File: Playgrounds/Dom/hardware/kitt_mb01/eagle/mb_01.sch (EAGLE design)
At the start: 50 parts, among them CON1 ARDUINO_UNO, CON2 KITT.DB01, IC1 LA5744TP, IC2.00 BQ24266RGET

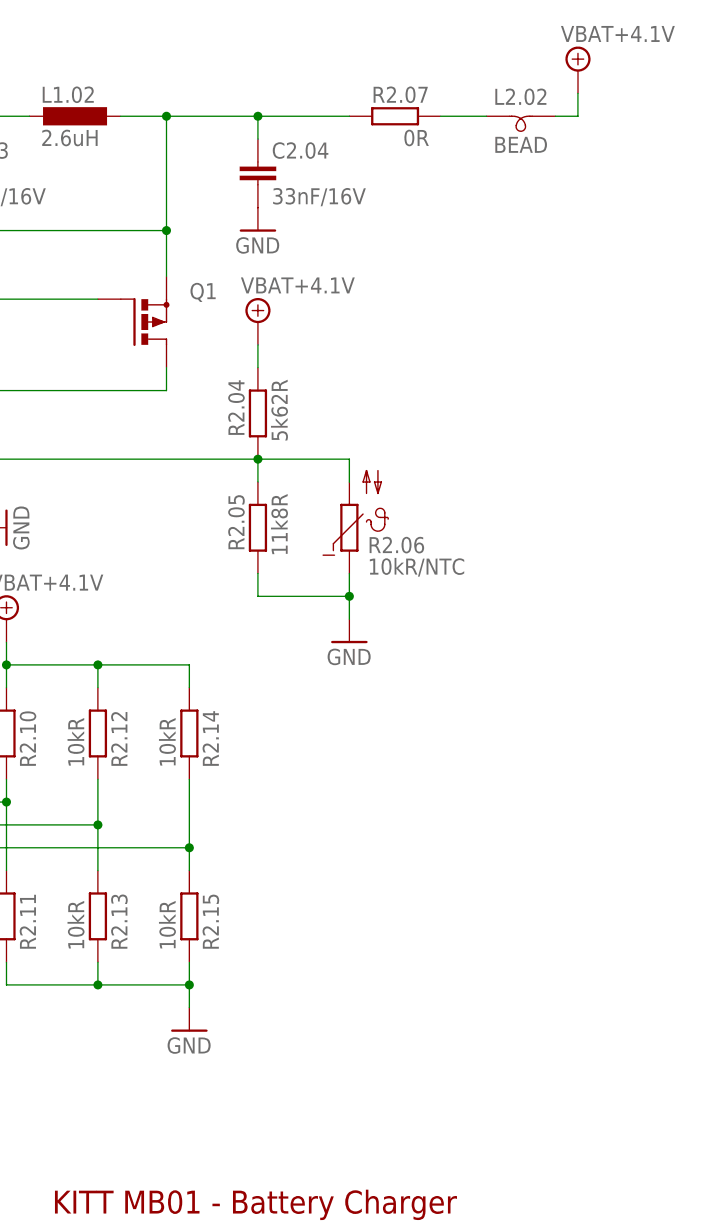
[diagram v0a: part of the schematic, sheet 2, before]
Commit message: did some more work on copying the charger layout
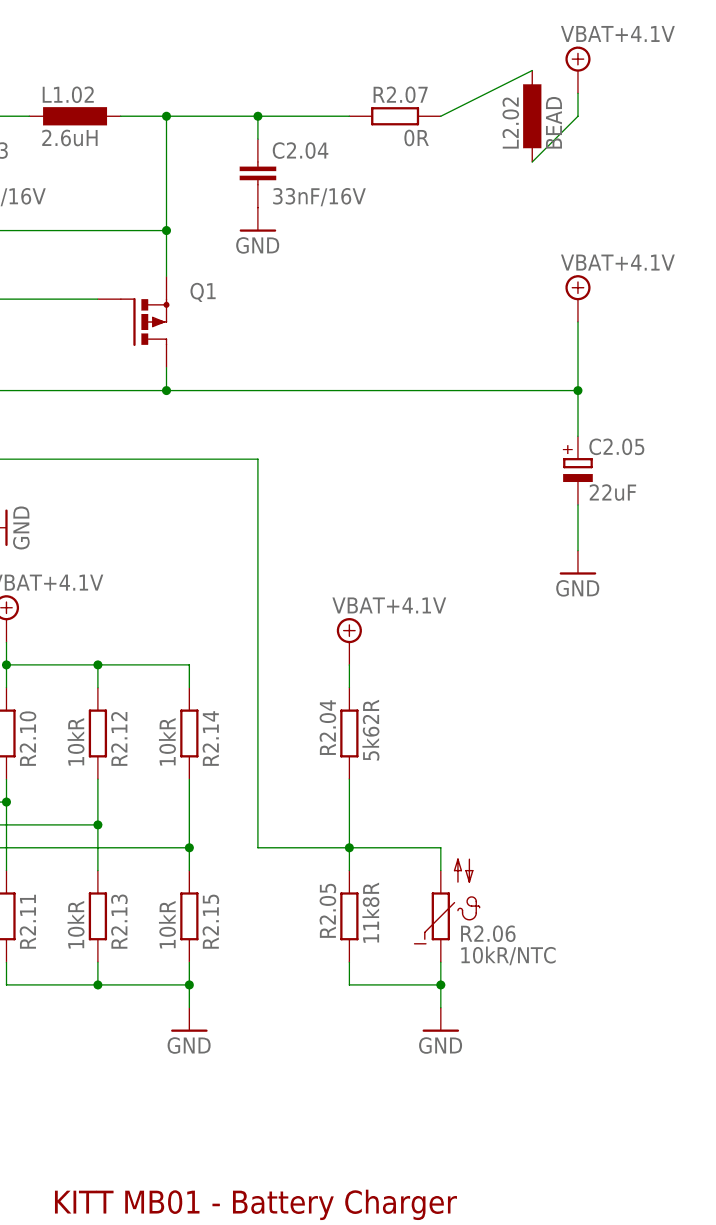
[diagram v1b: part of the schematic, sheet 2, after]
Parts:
- added C2.05: 22uF, rcl:CPOL-EUA/3216-18R
- C2.03: device rcl:C-EUC0805 -> rcl:C-EUC0603
- L2.02: device inductor-neosid:SM-B5 -> rcl:L-EUL2012C
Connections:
- removed net N$17: IC2.00PINS.BAT@1, IC2.00PINS.BAT@2, Q1.D
- net +4.1V: now also C2.05.+, IC2.00PINS.BAT@1, IC2.00PINS.BAT@2, Q1.D
- net GND: now also C2.05.-
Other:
- moved on the sheet: R2.04, R2.05, R2.06
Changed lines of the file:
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@@
 <part name="GND11" library="supply1" deviceset="GND" device=""/>
 <part name="L1.02" library="rcl" deviceset="L-EU" device="WE-TPC" value="2.6uH"/>
-<part name="C2.03" library="rcl" deviceset="C-EU" device="C0805" value="33nF/16V"/>
+<part name="C2.03" library="rcl" deviceset="C-EU" device="C0603" value="33nF/16V"/>
 <part name="Q1" library="transistor-power" deviceset="P-MOSFET-SO8" device=""/>
 <part name="SUPPLY1" library="supply2" deviceset="+4.1V" device="" value="VBAT+4.1V"/>
@@
 <part name="C2.04" library="rcl" deviceset="C-EU" device="C0805" value="33nF/16V"/>
 <part name="GND13" library="supply1" deviceset="GND" device=""/>
-<part name="L2.02" library="inductor-neosid" deviceset="SM-B" device="5" value="BEAD"/>
+<part name="L2.02" library="rcl" deviceset="L-EU" device="L2012C" value="BEAD"/>
 <part name="R2.07" library="rcl" deviceset="R-EU_" device="R0402" value="0R"/>
 <part name="GND14" library="supply1" deviceset="GND" device=""/>
@@
 <part name="GND15" library="supply1" deviceset="GND" device=""/>
 <part name="REF5" library="kitt.refs" deviceset="REF.GHOSTCAR.BCP" device=""/>
+<part name="C2.05" library="rcl" deviceset="CPOL-EU" device="A/3216-18R" value="22uF"/>
+<part name="GND16" library="supply1" deviceset="GND" device=""/>
+<part name="SUPPLY4" library="supply2" deviceset="+4.1V" device="" value="VBAT+4.1V"/>
 </parts>
 <sheets>
@@
 <instance part="SUPPLY1" gate="P" x="220.98" y="147.32"/>
 <instance part="R2.03" gate="G$1" x="147.32" y="96.52" rot="MR0"/>
-<instance part="R2.04" gate="G$1" x="185.42" y="109.22" rot="MR270"/>
-<instance part="R2.05" gate="G$1" x="185.42" y="96.52" rot="MR270"/>
-<instance part="R2.06" gate="1" x="195.58" y="96.52"/>
-<instance part="GND12" gate="1" x="195.58" y="83.82"/>
-<instance part="SUPPLY2" gate="P" x="185.42" y="119.38"/>
+<instance part="R2.04" gate="G$1" x="195.58" y="73.66" rot="MR270"/>
+<instance part="R2.05" gate="G$1" x="195.58" y="53.34" rot="MR270"/>
+<instance part="R2.06" gate="1" x="205.74" y="53.34"/>
+<instance part="GND12" gate="1" x="205.74" y="40.64"/>
+<instance part="SUPPLY2" gate="P" x="195.58" y="83.82"/>
 <instance part="C2.04" gate="G$1" x="185.42" y="137.16"/>
 <instance part="GND13" gate="1" x="185.42" y="129.54"/>
@@
 <instance part="GND15" gate="1" x="177.8" y="40.64"/>
 <instance part="REF5" gate="G$1" x="7.62" y="15.24"/>
+<instance part="C2.05" gate="G$1" x="220.98" y="104.14"/>
+<instance part="GND16" gate="1" x="220.98" y="91.44"/>
+<instance part="SUPPLY4" gate="P" x="220.98" y="121.92"/>
 </instances>
 <busses>
@@
 <segment>
 <pinref part="R2.05" gate="G$1" pin="2"/>
-<wire x1="185.42" y1="91.44" x2="185.42" y2="88.9" width="0.1524" layer="91"/>
-<wire x1="185.42" y1="88.9" x2="195.58" y2="88.9" width="0.1524" layer="91"/>
+<wire x1="195.58" y1="48.26" x2="195.58" y2="45.72" width="0.1524" layer="91"/>
+<wire x1="195.58" y1="45.72" x2="205.74" y2="45.72" width="0.1524" layer="91"/>
 <pinref part="GND12" gate="1" pin="GND"/>
-<wire x1="195.58" y1="88.9" x2="195.58" y2="86.36" width="0.1524" layer="91"/>
+<wire x1="205.74" y1="45.72" x2="205.74" y2="43.18" width="0.1524" layer="91"/>
 <pinref part="R2.06" gate="1" pin="1"/>
-<wire x1="195.58" y1="91.44" x2="195.58" y2="88.9" width="0.1524" layer="91"/>
-<junction x="195.58" y="88.9"/>
+<wire x1="205.74" y1="48.26" x2="205.74" y2="45.72" width="0.1524" layer="91"/>
+<junction x="205.74" y="45.72"/>
 </segment>
 <segment>
@@
 <junction x="167.64" y="45.72"/>
 </segment>
+<segment>
+<pinref part="C2.05" gate="G$1" pin="-"/>
+<pinref part="GND16" gate="1" pin="GND"/>
+<wire x1="220.98" y1="93.98" x2="220.98" y2="99.06" width="0.1524" layer="91"/>
+</segment>
 </net>
 <net name="N$8" class="0">
@@
 </segment>
 </net>
-<net name="N$17" class="0">
-<segment>
-<pinref part="Q1" gate="G$1" pin="D"/>
-<pinref part="IC2.00" gate="PINS" pin="BAT@2"/>
-<wire x1="175.26" y1="114.3" x2="175.26" y2="111.76" width="0.1524" layer="91"/>
-<wire x1="175.26" y1="111.76" x2="144.78" y2="111.76" width="0.1524" layer="91"/>
-<pinref part="IC2.00" gate="PINS" pin="BAT@1"/>
-<wire x1="144.78" y1="111.76" x2="139.7" y2="111.76" width="0.1524" layer="91"/>
-<wire x1="139.7" y1="114.3" x2="144.78" y2="114.3" width="0.1524" layer="91"/>
-<wire x1="144.78" y1="114.3" x2="144.78" y2="111.76" width="0.1524" layer="91"/>
-<junction x="144.78" y="111.76"/>
-</segment>
-</net>
 <net name="+4.1V" class="0">
 <segment>
 <pinref part="R2.04" gate="G$1" pin="1"/>
 <pinref part="SUPPLY2" gate="P" pin="+4.1V"/>
-<wire x1="185.42" y1="116.84" x2="185.42" y2="114.3" width="0.1524" layer="91"/>
+<wire x1="195.58" y1="81.28" x2="195.58" y2="78.74" width="0.1524" layer="91"/>
 </segment>
 <segment>
 <pinref part="L2.02" gate="G$1" pin="2"/>
 <pinref part="SUPPLY1" gate="P" pin="+4.1V"/>
-<wire x1="218.44" y1="142.24" x2="220.98" y2="142.24" width="0.1524" layer="91"/>
+<wire x1="215.9" y1="137.16" x2="220.98" y2="142.24" width="0.1524" layer="91"/>
 <wire x1="220.98" y1="142.24" x2="220.98" y2="144.78" width="0.1524" layer="91"/>
 </segment>
@@
 <junction x="167.64" y="81.28"/>
 </segment>
+<segment>
+<pinref part="Q1" gate="G$1" pin="D"/>
+<pinref part="IC2.00" gate="PINS" pin="BAT@2"/>
+<wire x1="175.26" y1="114.3" x2="175.26" y2="111.76" width="0.1524" layer="91"/>
+<wire x1="175.26" y1="111.76" x2="144.78" y2="111.76" width="0.1524" layer="91"/>
+<pinref part="IC2.00" gate="PINS" pin="BAT@1"/>
+<wire x1="144.78" y1="111.76" x2="139.7" y2="111.76" width="0.1524" layer="91"/>
+<wire x1="139.7" y1="114.3" x2="144.78" y2="114.3" width="0.1524" layer="91"/>
+<wire x1="144.78" y1="114.3" x2="144.78" y2="111.76" width="0.1524" layer="91"/>
+<junction x="144.78" y="111.76"/>
+<wire x1="175.26" y1="111.76" x2="220.98" y2="111.76" width="0.1524" layer="91"/>
+<junction x="175.26" y="111.76"/>
+<wire x1="220.98" y1="111.76" x2="220.98" y2="119.38" width="0.1524" layer="91"/>
+<pinref part="C2.05" gate="G$1" pin="+"/>
+<wire x1="220.98" y1="106.68" x2="220.98" y2="111.76" width="0.1524" layer="91"/>
+<junction x="220.98" y="111.76"/>
+<pinref part="SUPPLY4" gate="P" pin="+4.1V"/>
+</segment>
 </net>
 <net name="N$15" class="0">
@@
 <pinref part="R2.04" gate="G$1" pin="2"/>
 <wire x1="139.7" y1="104.14" x2="185.42" y2="104.14" width="0.1524" layer="91"/>
+<wire x1="185.42" y1="104.14" x2="185.42" y2="60.96" width="0.1524" layer="91"/>
 <pinref part="R2.05" gate="G$1" pin="1"/>
-<wire x1="185.42" y1="101.6" x2="185.42" y2="104.14" width="0.1524" layer="91"/>
-<junction x="185.42" y="104.14"/>
+<wire x1="195.58" y1="58.42" x2="195.58" y2="60.96" width="0.1524" layer="91"/>
 <pinref part="R2.06" gate="1" pin="2"/>
-<wire x1="185.42" y1="104.14" x2="195.58" y2="104.14" width="0.1524" layer="91"/>
-<wire x1="195.58" y1="104.14" x2="195.58" y2="101.6" width="0.1524" layer="91"/>
+<wire x1="195.58" y1="60.96" x2="195.58" y2="68.58" width="0.1524" layer="91"/>
+<wire x1="205.74" y1="60.96" x2="205.74" y2="58.42" width="0.1524" layer="91"/>
+<wire x1="185.42" y1="60.96" x2="195.58" y2="60.96" width="0.1524" layer="91"/>
+<junction x="195.58" y="60.96"/>
+<wire x1="195.58" y1="60.96" x2="205.74" y2="60.96" width="0.1524" layer="91"/>
 </segment>
 </net>
@@
 <pinref part="R2.07" gate="G$1" pin="1"/>
 <pinref part="L2.02" gate="G$1" pin="1"/>
-<wire x1="205.74" y1="142.24" x2="210.82" y2="142.24" width="0.1524" layer="91"/>
-</segment>
-</net>
+<wire x1="205.74" y1="142.24" x2="215.9" y2="147.32" width="0.1524" layer="91"/>
+</segment>
+</net>

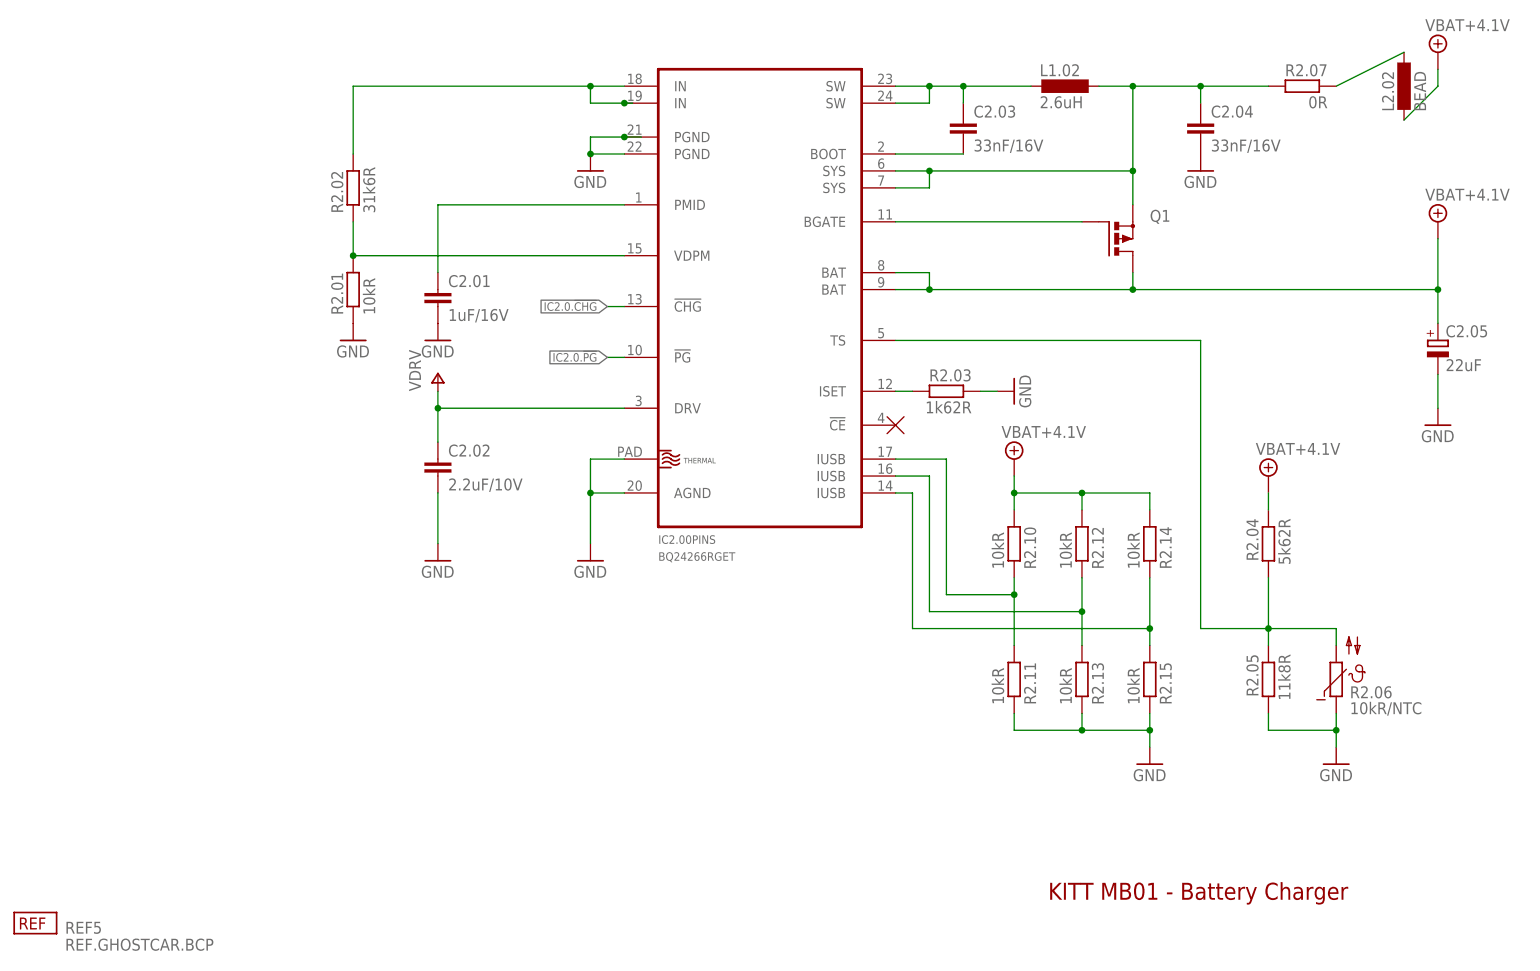
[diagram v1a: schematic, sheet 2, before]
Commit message: finished up on the charger circuit, roughly...
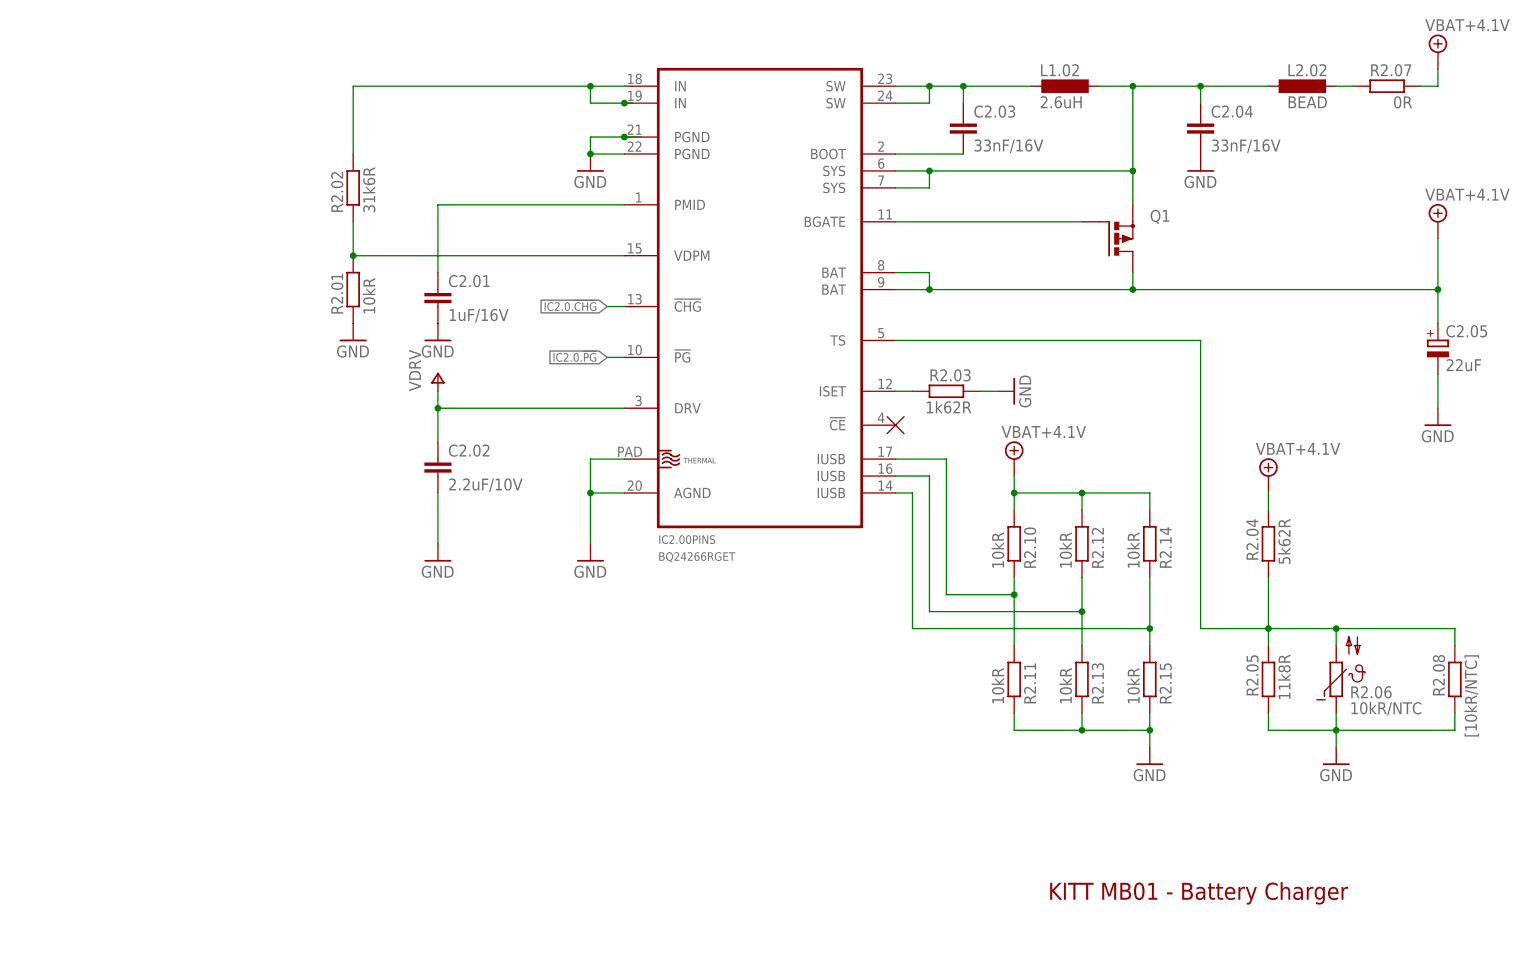
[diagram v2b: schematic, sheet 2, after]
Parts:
- removed REF5: REF.GHOSTCAR.BCP, kitt.refs:REF.GHOSTCAR.BCP
- added R2.08: [10kR/NTC], rcl:R-EU_R0402
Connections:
- net +4.1V: now also R2.07.1; no longer L2.02.2
- net GND: now also R2.08.2
- net N$15: now also R2.08.1
- net N$16: now also L2.02.2, R2.07.2; no longer L2.02.1, R2.07.1
- net N$18: now also L2.02.1; no longer R2.07.2
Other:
- moved on the sheet: L2.02, R2.07
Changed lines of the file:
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@@
 <part name="SUPPLY3" library="supply2" deviceset="+4.1V" device="" value="VBAT+4.1V"/>
 <part name="GND15" library="supply1" deviceset="GND" device=""/>
-<part name="REF5" library="kitt.refs" deviceset="REF.GHOSTCAR.BCP" device=""/>
 <part name="C2.05" library="rcl" deviceset="CPOL-EU" device="A/3216-18R" value="22uF"/>
 <part name="GND16" library="supply1" deviceset="GND" device=""/>
 <part name="SUPPLY4" library="supply2" deviceset="+4.1V" device="" value="VBAT+4.1V"/>
+<part name="R2.08" library="rcl" deviceset="R-EU_" device="R0402" value="[10kR/NTC]"/>
 </parts>
 <sheets>
@@
 <instance part="C2.04" gate="G$1" x="185.42" y="137.16"/>
 <instance part="GND13" gate="1" x="185.42" y="129.54"/>
-<instance part="L2.02" gate="G$1" x="215.9" y="142.24"/>
-<instance part="R2.07" gate="G$1" x="200.66" y="142.24" rot="MR0"/>
+<instance part="L2.02" gate="G$1" x="200.66" y="142.24" rot="MR270"/>
+<instance part="R2.07" gate="G$1" x="213.36" y="142.24" rot="MR0"/>
 <instance part="GND14" gate="1" x="157.48" y="96.52" rot="R90"/>
 <instance part="R2.10" gate="G$1" x="157.48" y="73.66" rot="MR90"/>
@@
 <instance part="SUPPLY3" gate="P" x="157.48" y="86.36"/>
 <instance part="GND15" gate="1" x="177.8" y="40.64"/>
-<instance part="REF5" gate="G$1" x="7.62" y="15.24"/>
 <instance part="C2.05" gate="G$1" x="220.98" y="104.14"/>
 <instance part="GND16" gate="1" x="220.98" y="91.44"/>
 <instance part="SUPPLY4" gate="P" x="220.98" y="121.92"/>
+<instance part="R2.08" gate="G$1" x="223.52" y="53.34" rot="MR270"/>
 </instances>
 <busses>
@@
 <wire x1="205.74" y1="48.26" x2="205.74" y2="45.72" width="0.1524" layer="91"/>
 <junction x="205.74" y="45.72"/>
+<pinref part="R2.08" gate="G$1" pin="2"/>
+<wire x1="223.52" y1="48.26" x2="223.52" y2="45.72" width="0.1524" layer="91"/>
+<wire x1="223.52" y1="45.72" x2="205.74" y2="45.72" width="0.1524" layer="91"/>
 </segment>
 <segment>
@@
 </segment>
 <segment>
-<pinref part="L2.02" gate="G$1" pin="2"/>
 <pinref part="SUPPLY1" gate="P" pin="+4.1V"/>
-<wire x1="215.9" y1="137.16" x2="220.98" y2="142.24" width="0.1524" layer="91"/>
 <wire x1="220.98" y1="142.24" x2="220.98" y2="144.78" width="0.1524" layer="91"/>
+<pinref part="R2.07" gate="G$1" pin="1"/>
+<wire x1="218.44" y1="142.24" x2="220.98" y2="142.24" width="0.1524" layer="91"/>
 </segment>
 <segment>
@@
 <junction x="195.58" y="60.96"/>
 <wire x1="195.58" y1="60.96" x2="205.74" y2="60.96" width="0.1524" layer="91"/>
+<pinref part="R2.08" gate="G$1" pin="1"/>
+<wire x1="223.52" y1="58.42" x2="223.52" y2="60.96" width="0.1524" layer="91"/>
+<wire x1="223.52" y1="60.96" x2="205.74" y2="60.96" width="0.1524" layer="91"/>
+<junction x="205.74" y="60.96"/>
 </segment>
 </net>
@@
 <wire x1="185.42" y1="142.24" x2="185.42" y2="139.7" width="0.1524" layer="91"/>
 <junction x="175.26" y="142.24"/>
-<pinref part="R2.07" gate="G$1" pin="2"/>
-<wire x1="185.42" y1="142.24" x2="195.58" y2="142.24" width="0.1524" layer="91"/>
+<pinref part="L2.02" gate="G$1" pin="1"/>
+<wire x1="195.58" y1="142.24" x2="185.42" y2="142.24" width="0.1524" layer="91"/>
 <junction x="185.42" y="142.24"/>
-</segment>
-</net>
-<net name="N$16" class="0">
-<segment>
-<pinref part="R2.07" gate="G$1" pin="1"/>
-<pinref part="L2.02" gate="G$1" pin="1"/>
-<wire x1="205.74" y1="142.24" x2="215.9" y2="147.32" width="0.1524" layer="91"/>
 </segment>
 </net>
@@
 </segment>
 </net>
+<net name="N$16" class="0">
+<segment>
+<pinref part="L2.02" gate="G$1" pin="2"/>
+<pinref part="R2.07" gate="G$1" pin="2"/>
+<wire x1="205.74" y1="142.24" x2="208.28" y2="142.24" width="0.1524" layer="91"/>
+</segment>
+</net>
